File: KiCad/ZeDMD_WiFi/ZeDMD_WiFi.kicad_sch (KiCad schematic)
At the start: 0 parts

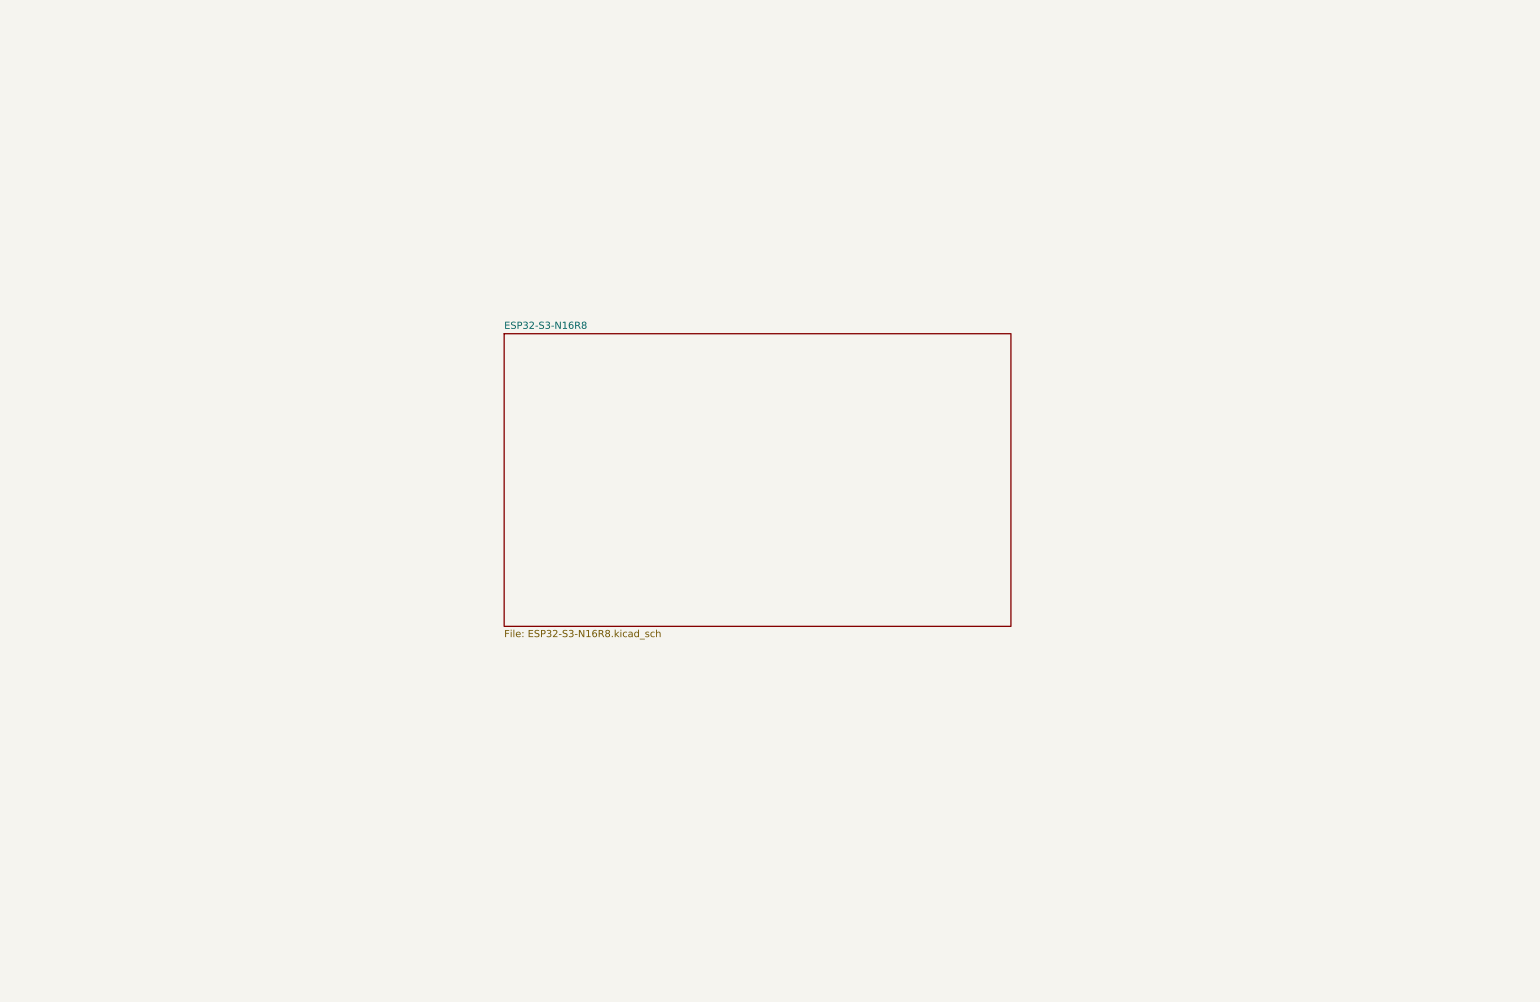
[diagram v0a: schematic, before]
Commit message: Initial setup
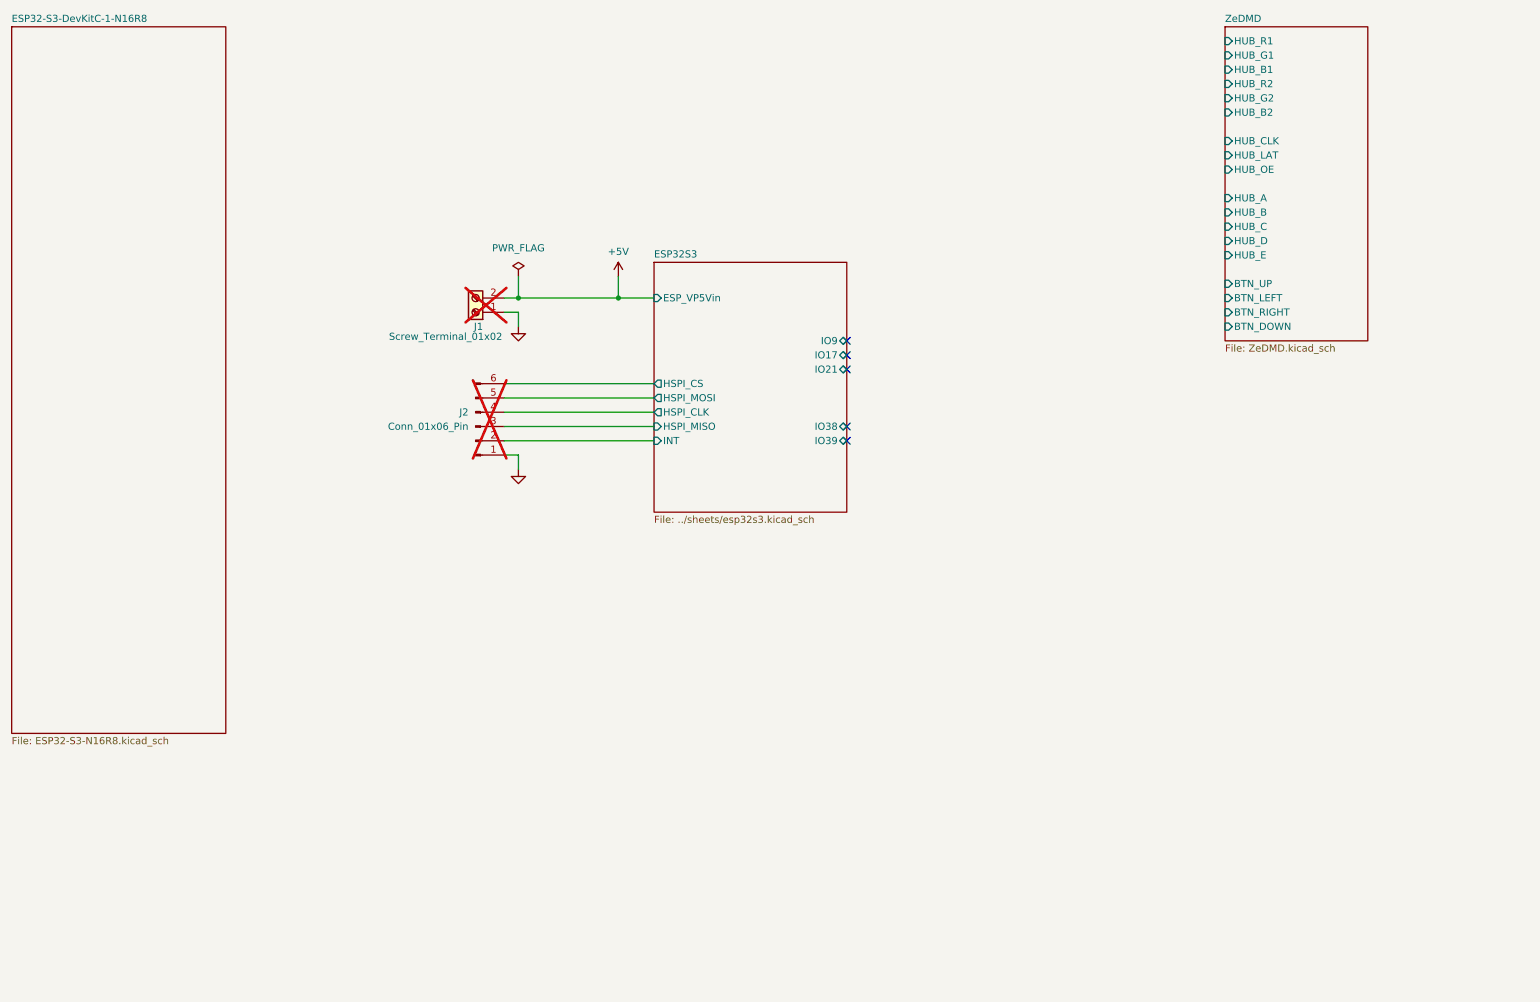
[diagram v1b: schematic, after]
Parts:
- added J1: Screw_Terminal_01x02, TerminalBlock_Phoenix:TerminalBlock_Phoenix_MKDS-1,5-2-5.08_1x02_P5.08mm_Horizontal, symbol Connector:Screw_Terminal_01x02
- added J2: Conn_01x06_Pin, Connector_PinHeader_2.54mm:PinHeader_1x06_P2.54mm_Vertical, symbol Connector:Conn_01x06_Pin
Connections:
- new net +5V: J1.2 (Pin_2)
- new net ESP32S3/HSPI_CLK: J2.4 (Pin_4)
- new net ESP32S3/HSPI_CS: J2.6 (Pin_6)
- new net ESP32S3/HSPI_MISO: J2.3 (Pin_3)
- new net ESP32S3/HSPI_MOSI: J2.5 (Pin_5)
- new net ESP32S3/INT: J2.2 (Pin_2)
- new net GND: J1.1 (Pin_1), J2.1 (Pin_1)
- no-connect marks 0 -> 5
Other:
- removed sheet ESP32-S3-N16R8
- added sheet ESP32-S3-DevKitC-1-N16R8 (ESP32-S3-N16R8.kicad_sch)
- added sheet ESP32S3 (../sheets/esp32s3.kicad_sch)
- added sheet ZeDMD (ZeDMD.kicad_sch)
- company: (none) -> elabree
- title: (none) -> ZeDMD ESP32-S3 (N16R8) basic

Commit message: SchematicsV1.1
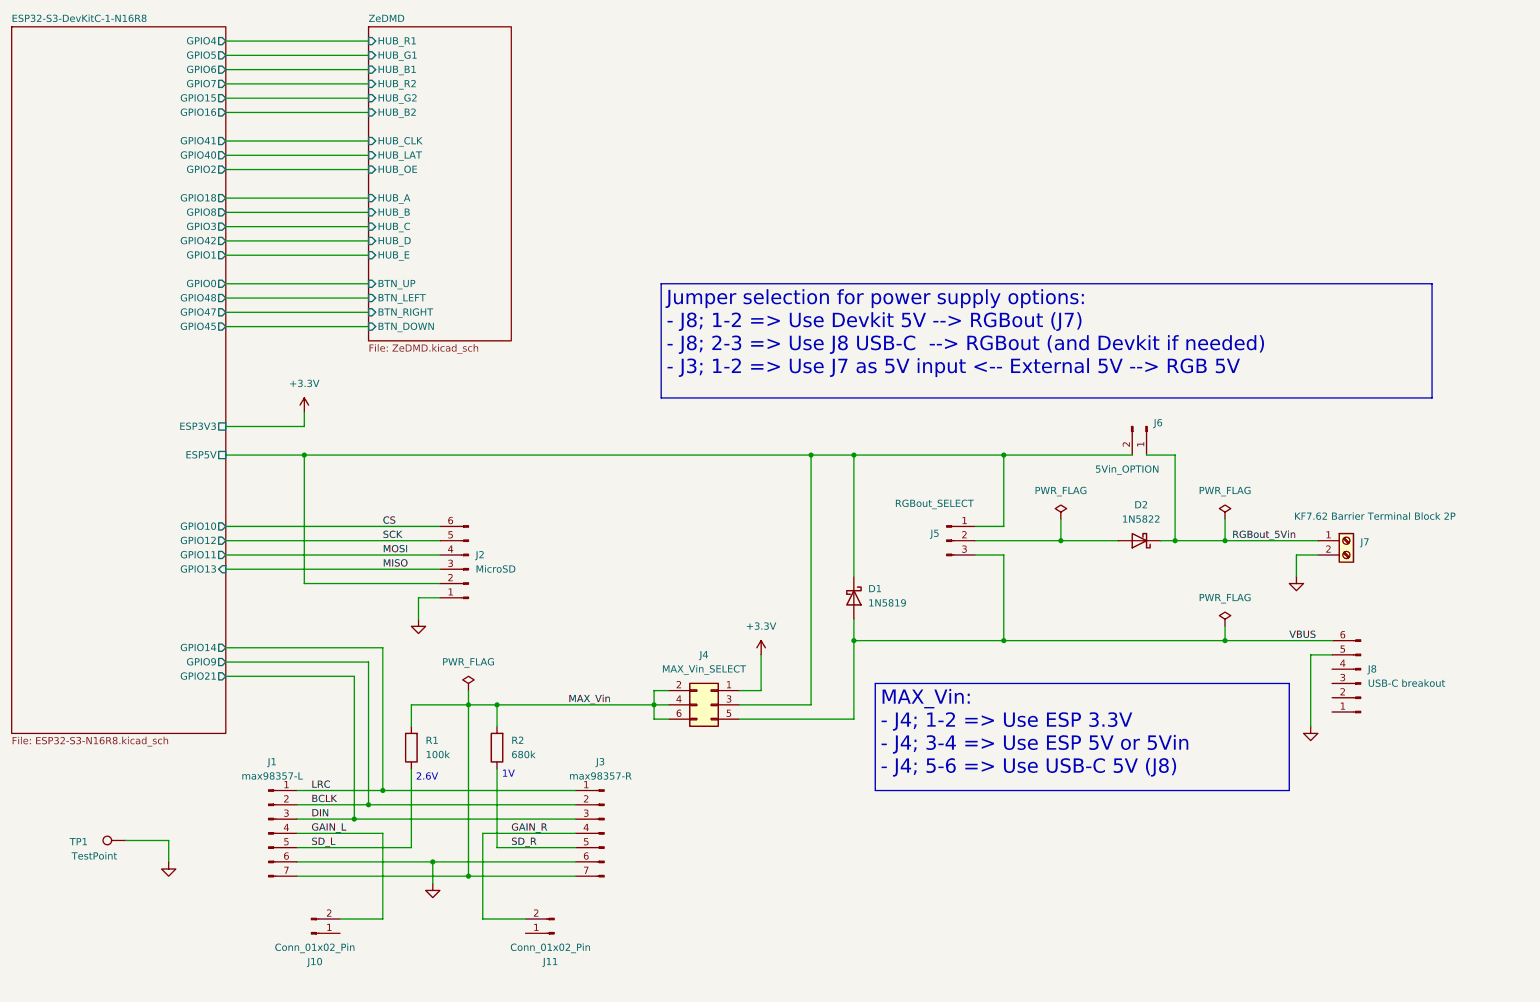
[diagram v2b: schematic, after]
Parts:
- removed J1: Screw_Terminal_01x02, TerminalBlock_Phoenix:TerminalBlock_Phoenix_MKDS-1,5-2-5.08_1x02_P5.08mm_Horizontal, symbol Connector:Screw_Terminal_01x02
- added D1: 1N5819, Diode_THT:D_DO-41_SOD81_P10.16mm_Horizontal, symbol Diode:1N5819
- added D2: 1N5822, Diode_THT:D_DO-201AD_P15.24mm_Horizontal, symbol Diode:1N5822
- added J1: max98357-L, Connector_PinSocket_2.54mm:PinSocket_1x07_P2.54mm_Vertical, symbol Connector:Conn_01x07_Pin
- added J10, J11: Conn_01x02_Pin, Connector_PinHeader_2.54mm:PinHeader_1x02_P2.54mm_Vertical, symbol Connector:Conn_01x02_Pin
- added J3: max98357-R, Connector_PinSocket_2.54mm:PinSocket_1x07_P2.54mm_Vertical, symbol Connector:Conn_01x07_Pin
- added J4: MAX_Vin_SELECT, Connector_PinHeader_2.54mm:PinHeader_2x03_P2.54mm_Vertical, symbol Connector_Generic:Conn_02x03_Odd_Even
- added J5: RGBout_SELECT, Connector_PinHeader_2.54mm:PinHeader_1x03_P2.54mm_Vertical, symbol Connector:Conn_01x03_Pin
- added J6: 5Vin_OPTION, Connector_PinHeader_2.54mm:PinHeader_1x02_P2.54mm_Vertical, symbol Connector:Conn_01x02_Pin
- added J7: KF7.62 Barrier Terminal Block 2P, ZeDMD_WiFi:KF7.62_2P, symbol Connector:Screw_Terminal_01x02
- added J8: USB-C breakout, Connector_PinSocket_2.54mm:PinSocket_1x06_P2.54mm_Vertical, symbol Connector:Conn_01x06_Pin
- added R1: 100k, Resistor_THT:R_Axial_DIN0207_L6.3mm_D2.5mm_P10.16mm_Horizontal, symbol Device:R
- added R2: 680k, Resistor_THT:R_Axial_DIN0207_L6.3mm_D2.5mm_P10.16mm_Horizontal, symbol Device:R
- added TP1: TestPoint, Connector_PinHeader_2.54mm:PinHeader_1x01_P2.54mm_Vertical, symbol Connector:TestPoint
- J2: value Conn_01x06_Pin -> MicroSD; footprint Connector_PinHeader_2.54mm:PinHeader_1x06_P2.54mm_Vertical -> Connector_PinSocket_2.54mm:PinSocket_1x06_P2.54mm_Vertical; now fitted
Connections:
- net GND: now also J1.6 (Pin_6), J3.6 (Pin_6), J7.2 (Pin_2), J8.5 (Pin_5), TP1.1
- net ESP32S3/HSPI_CLK renamed MOSI
- net ESP32S3/HSPI_CS renamed CS
- net ESP32S3/HSPI_MISO renamed MISO
- net ESP32S3/HSPI_MOSI renamed SCK
- net ESP32S3/INT renamed ESP32-S3-DevKitC-1-N16R8/ESP5V
- net ESP32-S3-DevKitC-1-N16R8/ESP5V: now also D1.1 (K), J4.3 (Pin_3), J5.1 (Pin_1), J6.2 (Pin_2)
- new net: D2.2 (A), J5.2 (Pin_2)
- new net +3.3V: J4.1 (Pin_1)
- new net BCLK: J1.2 (Pin_2), J3.2 (Pin_2)
- new net DIN: J1.3 (Pin_3), J3.3 (Pin_3)
- new net GAIN_L: J1.4 (Pin_4), J10.2 (Pin_2)
- new net GAIN_R: J11.2 (Pin_2), J3.4 (Pin_4)
- new net LRC: J1.1 (Pin_1), J3.1 (Pin_1)
- new net MAX_Vin: J1.7 (Pin_7), J3.7 (Pin_7), J4.2 (Pin_2), J4.4 (Pin_4), J4.6 (Pin_6), R1.2, R2.2
- new net RGBout_5Vin: D2.1 (K), J6.1 (Pin_1), J7.1 (Pin_1)
- new net SD_L: J1.5 (Pin_5), R1.1
- new net SD_R: J3.5 (Pin_5), R2.1
- new net VBUS: D1.2 (A), J4.5 (Pin_5), J5.3 (Pin_3), J8.6 (Pin_6)
- no-connect marks 5 -> 0
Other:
- removed sheet ESP32S3
- sheet ESP32-S3-DevKitC-1-N16R8 ports: added ESP3V3, ESP5V, GPIO0, GPIO1, GPIO10, GPIO11, GPIO12, GPIO13, GPIO14, GPIO15, GPIO16, GPIO18, GPIO2, GPIO21, GPIO3, GPIO4, GPIO40, GPIO41, GPIO42, GPIO45, GPIO47, GPIO48, GPIO5, GPIO6, GPIO7, GPIO8, GPIO9; removed none
- note added: "1V"
- note added: "2.6V"
- title: ZeDMD ESP32-S3 (N16R8) basic -> ZeDMD-WIFI-128x32

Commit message: Schematics update and pngs added
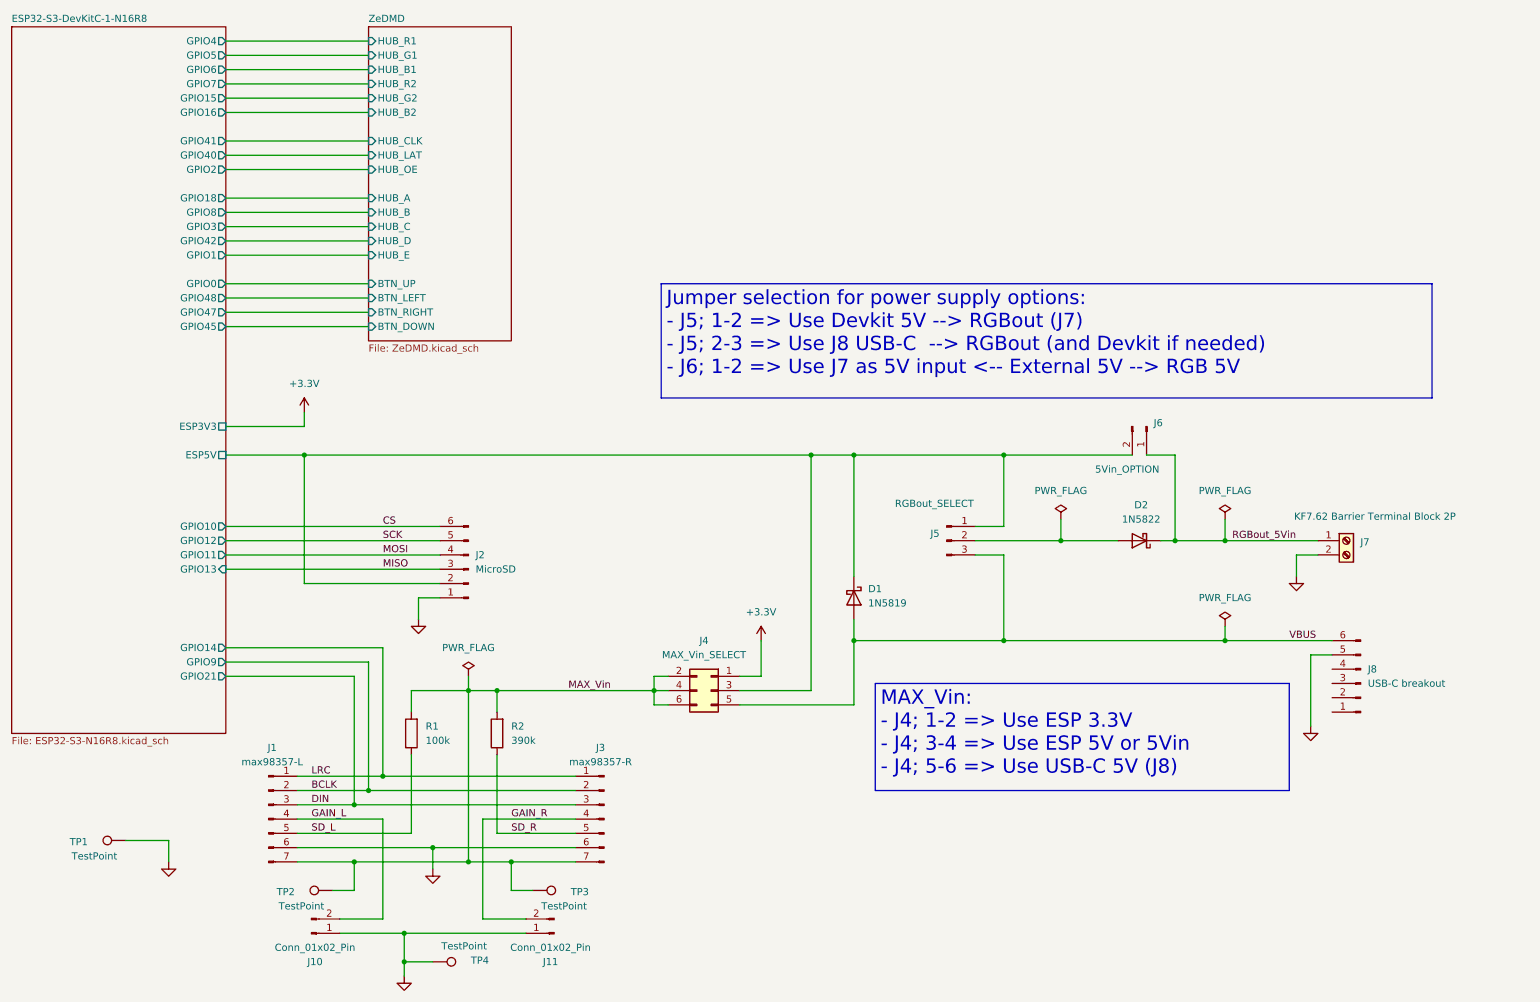
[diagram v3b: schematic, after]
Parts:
- added TP2, TP3, TP4: TestPoint, Connector_PinHeader_2.54mm:PinHeader_1x01_P2.54mm_Vertical, symbol Connector:TestPoint
- R2: value 680k -> 390k
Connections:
- net GND: now also J10.1 (Pin_1), J11.1 (Pin_1), TP4.1
- net MAX_Vin: now also TP2.1, TP3.1
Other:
- note removed: "1V"
- note removed: "2.6V"
- moved on the sheet: J1, J3, J4, R1, R2

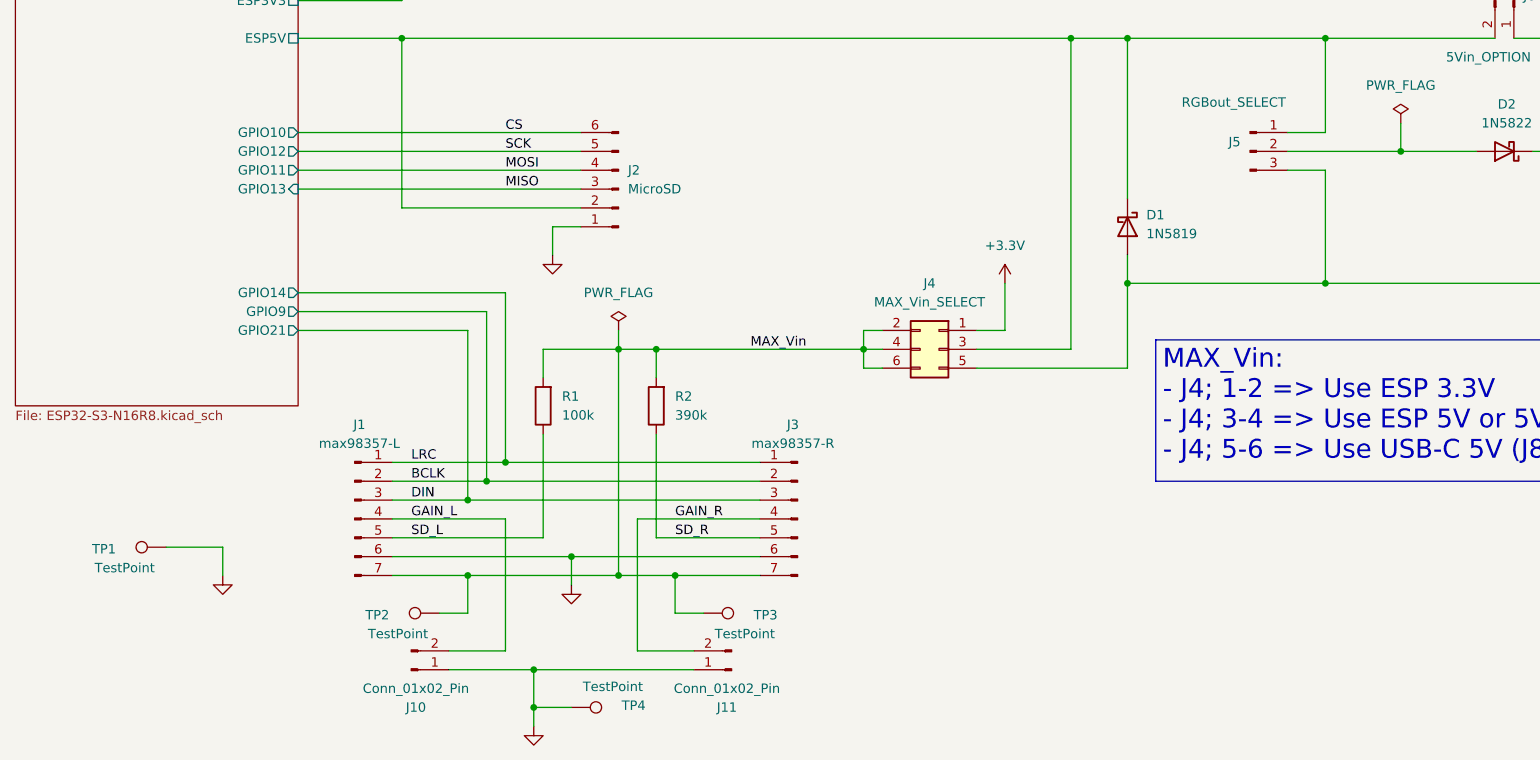
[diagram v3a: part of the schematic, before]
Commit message: Placement ready
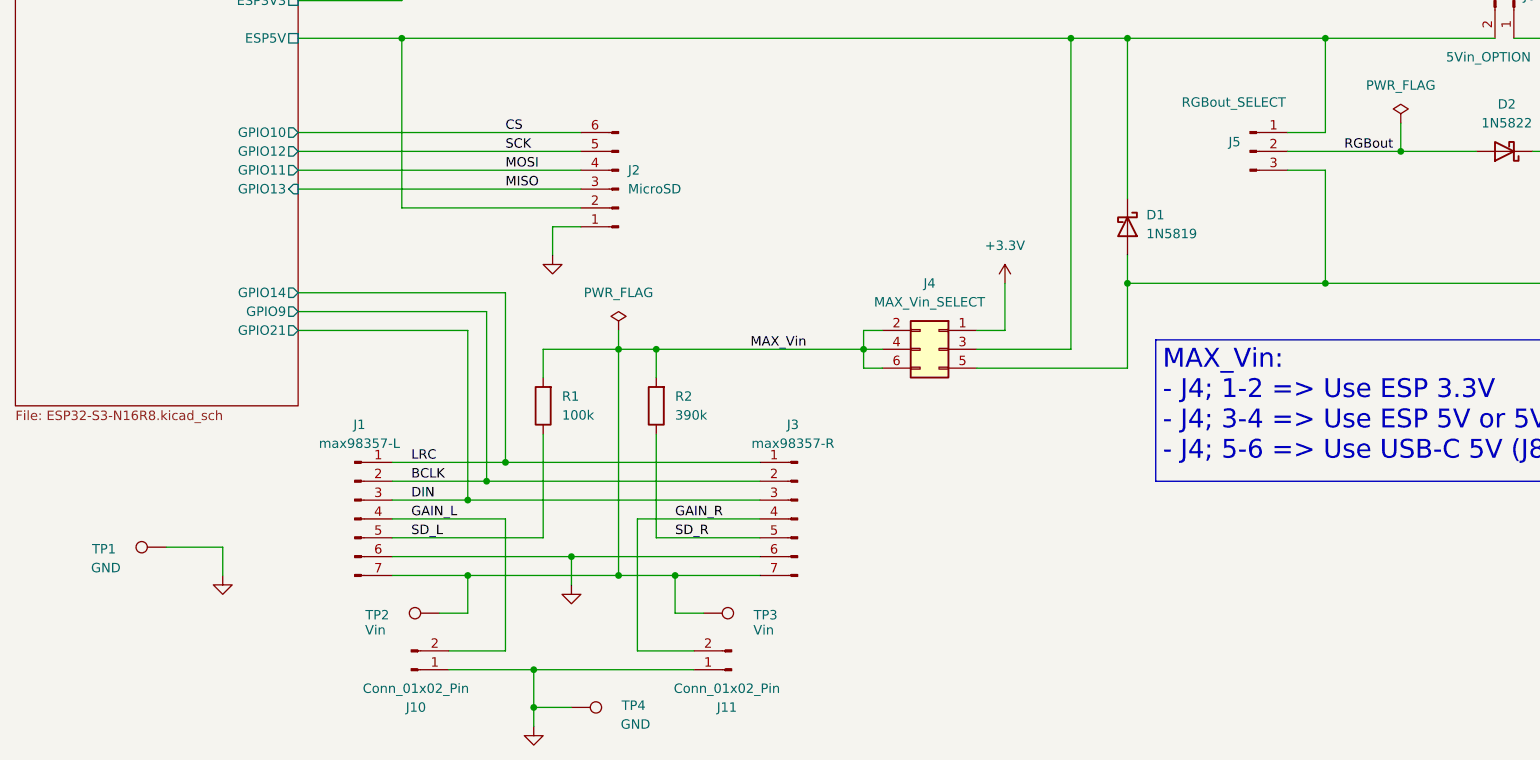
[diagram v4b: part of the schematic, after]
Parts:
- TP1, TP4: value TestPoint -> GND
- TP2, TP3: value TestPoint -> Vin
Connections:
- net RGBout: now reaches D2.2 (A), J5.2 (Pin_2)
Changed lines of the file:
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@@
 		)
 	)
+	(label "RGBout"
+		(at 204.47 116.84 0)
+		(effects
+			(font
+				(size 1.27 1.27)
+			)
+			(justify left bottom)
+		)
+	)
 	(label "SD_R"
 		(at 114.3 168.91 0)
@@
 			)
 		)
-		(property "Value" "TestPoint"
-			(at 40.132 172.974 90)
+		(property "Value" "GND"
+			(at 37.592 172.974 90)
 			(show_name no)
 			(do_not_autoplace no)
@@
 			)
 		)
-		(property "Value" "TestPoint"
-			(at 76.962 181.864 90)
+		(property "Value" "Vin"
+			(at 73.914 181.356 90)
 			(show_name no)
 			(do_not_autoplace no)
@@
 			)
 		)
-		(property "Value" "TestPoint"
-			(at 105.918 188.976 90)
+		(property "Value" "GND"
+			(at 108.966 194.056 90)
 			(show_name no)
 			(do_not_autoplace no)
@@
 			)
 		)
-		(property "Value" "TestPoint"
-			(at 123.698 181.864 90)
+		(property "Value" "Vin"
+			(at 126.238 181.356 90)
 			(show_name no)
 			(do_not_autoplace no)
